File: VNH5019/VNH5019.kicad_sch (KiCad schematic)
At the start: 17 parts, among them Q2 FCD600N60Z, SW2 HAD-04H-R, U5 VNH5019A-E

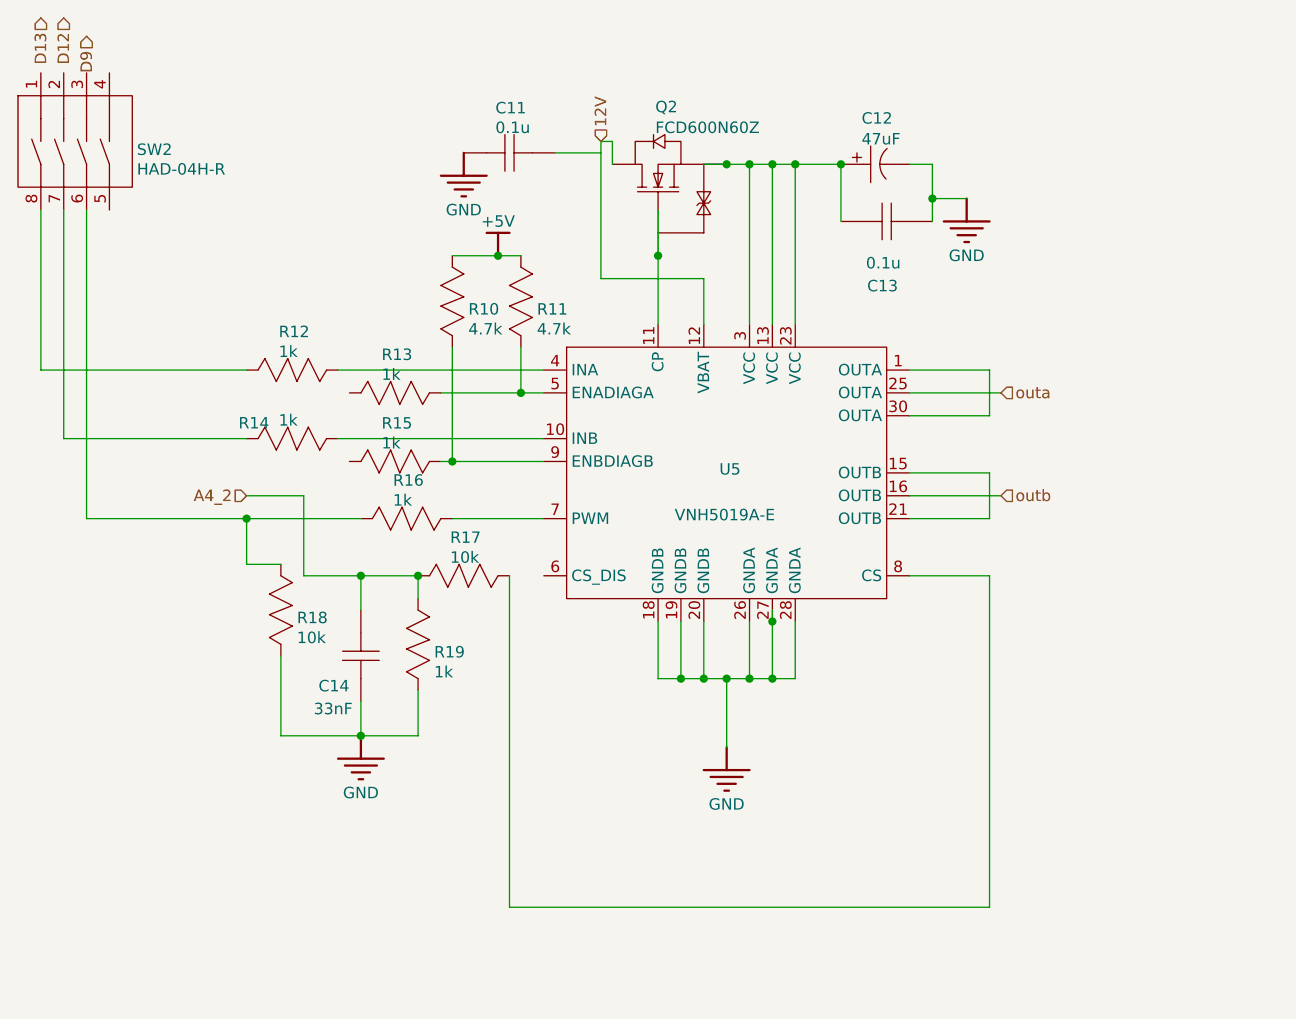
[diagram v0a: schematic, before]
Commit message: pcbv1.0
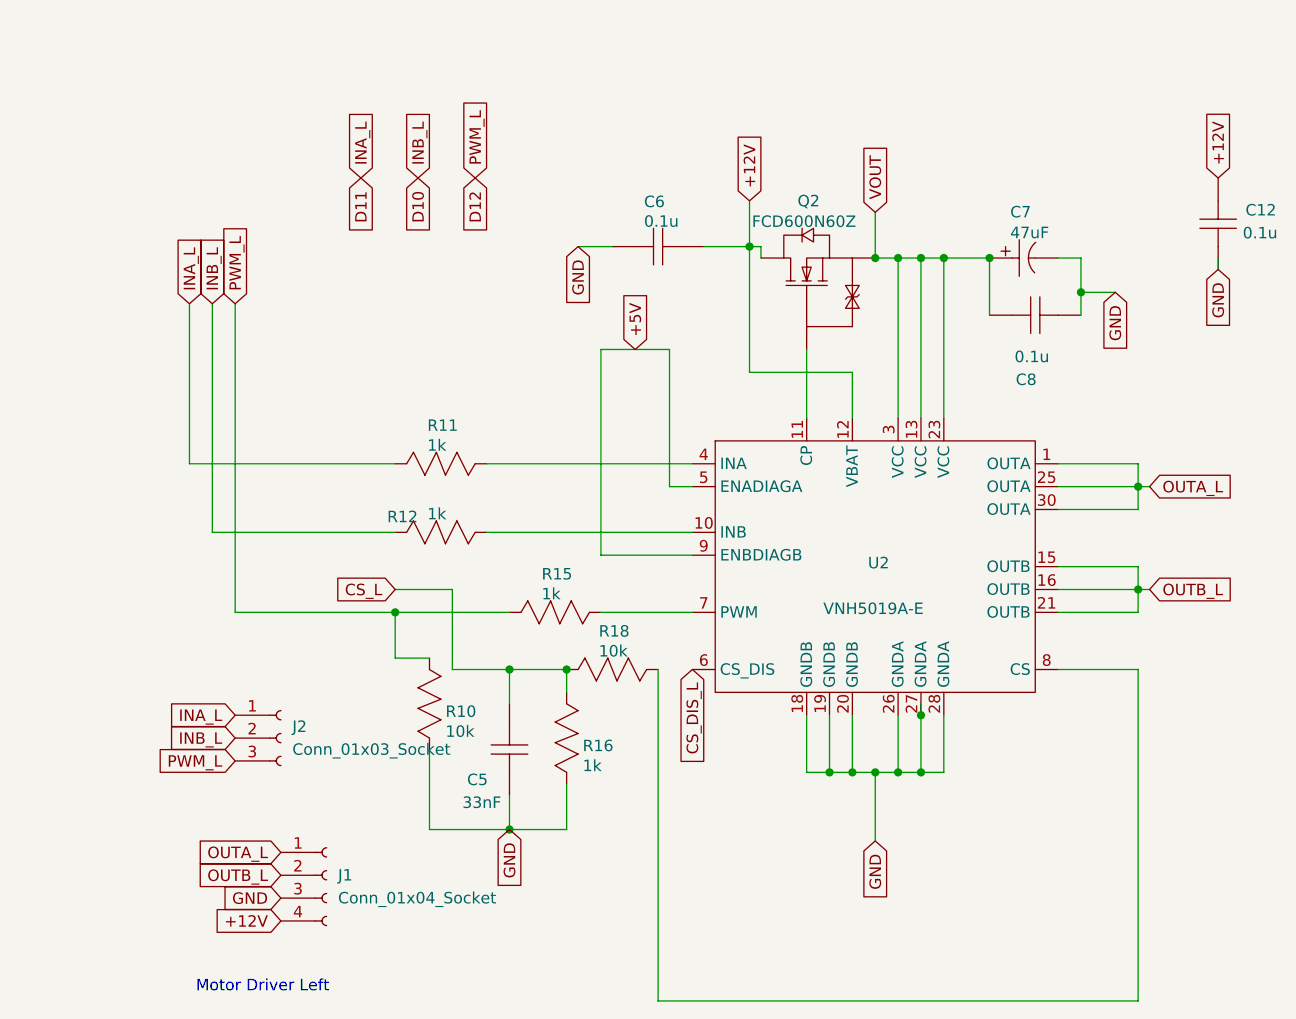
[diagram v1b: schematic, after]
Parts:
- removed C11, C13: 0.1u, symbol VNH5019-altium-import:root_0_0.1u_
- removed C12: 47uF, symbol VNH5019-altium-import:root_0_47uF_
- removed C14: 33nF, symbol VNH5019-altium-import:root_3_33nF_
- removed R10, R11: 4.7k, symbol VNH5019-altium-import:root_1_4.7k_
- removed R13, R14, R16: 1k, symbol VNH5019-altium-import:root_0_1k_
- removed R17: 10k, symbol VNH5019-altium-import:root_0_10k_
- removed R18: 10k, symbol VNH5019-altium-import:root_1_10k_
- removed R19: 1k, symbol VNH5019-altium-import:root_1_1k_
- removed SW2: HAD-04H-R, symbol VNH5019-altium-import:root_0_HAD-04H-R_
- removed U5: VNH5019A-E, symbol VNH5019-altium-import:root_0_VNH5019A-E_
- added C12, C6, C8: 0.1u, Capacitor_SMD:C_0805_2012Metric, symbol VNH5019-altium-import:root_0_0.1u_
- added C5: 33nF, Capacitor_SMD:C_0805_2012Metric, symbol VNH5019-altium-import:root_3_33nF_
- added C7: 47uF, Capacitor_SMD:C_Elec_6.3x5.4, symbol VNH5019-altium-import:root_0_47uF_
- added J1: Conn_01x04_Socket, Connector_PinSocket_2.54mm:PinSocket_1x04_P2.54mm_Vertical, symbol Connector:Conn_01x04_Socket
- added J2: Conn_01x03_Socket, Connector_PinSocket_2.54mm:PinSocket_1x03_P2.54mm_Vertical, symbol Connector:Conn_01x03_Socket
- added R10: 10k, Resistor_SMD:R_0508_1220Metric, symbol VNH5019-altium-import:root_1_10k_
- added R11: 1k, Resistor_SMD:R_0508_1220Metric, symbol VNH5019-altium-import:root_0_1k_
- added R16: 1k, Resistor_SMD:R_0508_1220Metric, symbol VNH5019-altium-import:root_1_1k_
- added R18: 10k, Resistor_SMD:R_0508_1220Metric, symbol VNH5019-altium-import:root_0_10k_
- added U2: VNH5019A-E, Package_SO:ST_MultiPowerSO-30, symbol VNH5019-altium-import:root_0_VNH5019A-E_
- Q2: footprint (none) -> Package_TO_SOT_SMD:TO-252-2
- R12, R15: footprint (none) -> Resistor_SMD:R_0508_1220Metric
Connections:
- net +5V: now also U2.5 (ENADIAGA), U2.9 (ENBDIAGB)
- net D12: now also R15.1, J2.3 (Pin_3), R10.2
- net GND: now also C12.2, C5.2, C6.1, C7.2, C8.2, J1.3 (Pin_3), R10.1, R16.1, U2.18 (GNDB), U2.19 (GNDB), U2.20 (GNDB), U2.26 (GNDA), U2.27 (GNDA), U2.28 (GNDA)
- net at R15.2: now also U2.7 (PWM)
- net at Q2.1 (G): now also U2.11 (CP)
- net VOUT: now reaches Q2.3 (S)
- net VOUT: now also C7.1, C8.1, U2.13 (VCC), U2.23 (VCC), U2.3 (VCC)
- net at R12.2: now also U2.10 (INB)
- net D10: now reaches R12.1
- net D10: now also J2.2 (Pin_2)
- removed net 12V: Q2.4 (D)
- new net: R18.2, U2.8 (CS)
- new net: R11.2, U2.4 (INA)
- new net +12V: C12.1, C6.2, J1.4 (Pin_4), Q2.2 (D), U2.12 (VBAT)
- new net CS_DIS_L: U2.6 (CS_DIS)
- new net CS_L: C5.1, R16.2, R18.1
- new net D11: J2.1 (Pin_1), R11.1
- new net OUTA_L: J1.1 (Pin_1), U2.1 (OUTA), U2.25 (OUTA), U2.30 (OUTA)
- new net OUTB_L: J1.2 (Pin_2), U2.15 (OUTB), U2.16 (OUTB), U2.21 (OUTB)
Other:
- note added: "Motor Driver Left"
